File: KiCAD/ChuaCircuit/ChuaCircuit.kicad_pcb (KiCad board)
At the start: 2 copper layers, 30 x 40 mm, 21 parts, among them X1 TP3, Y1 TP2

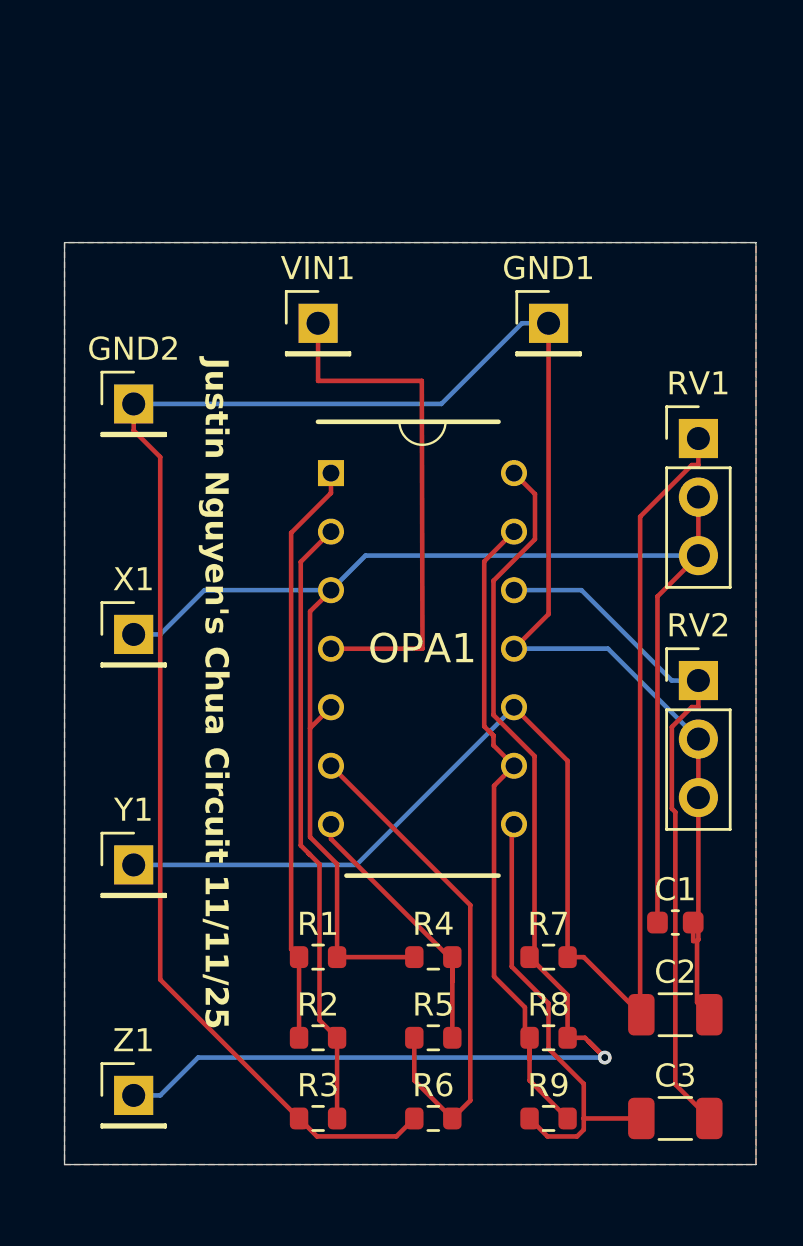
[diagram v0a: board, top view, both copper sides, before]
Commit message: Completed routing and the pcb design but need to make GND plane
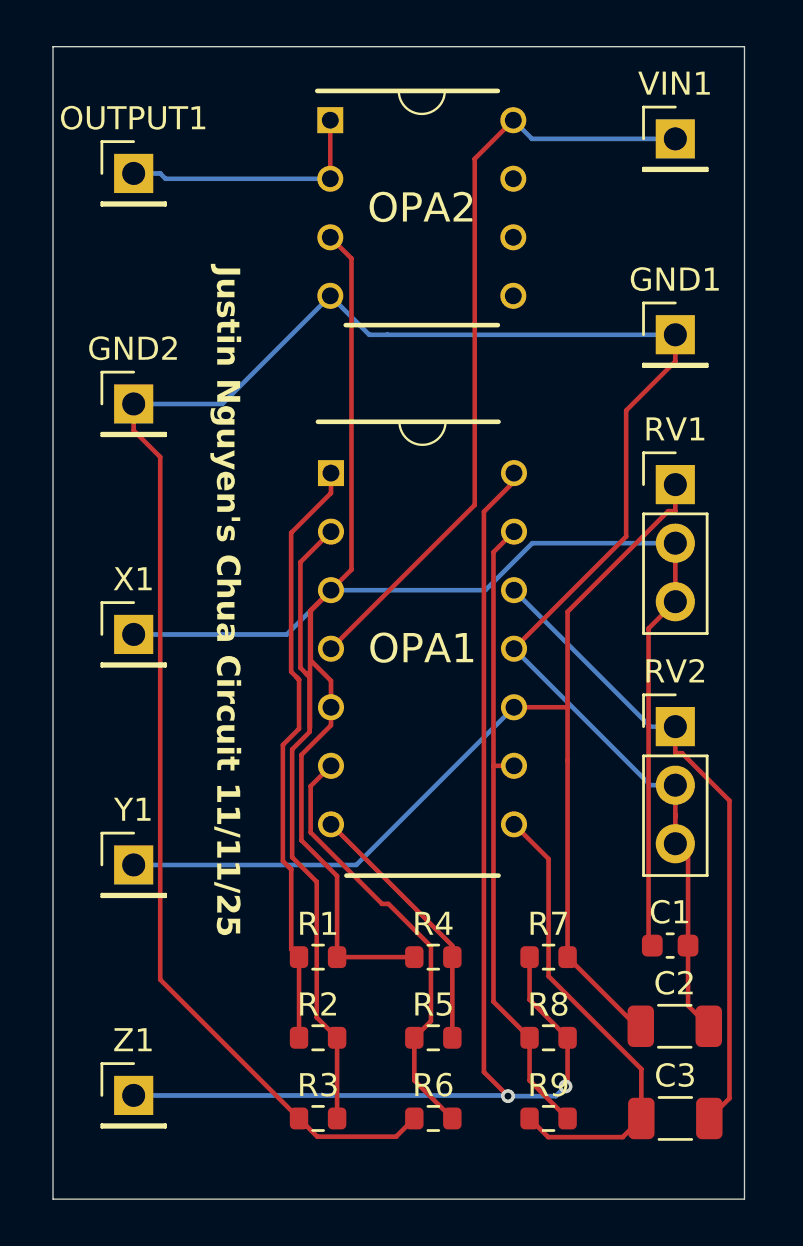
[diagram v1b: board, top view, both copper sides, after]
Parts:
- added OPA2: TL082, SamacSys_Parts:TL082, F.Cu at (138.5, 83.5)
- added OUTPUT1: Male_Header_1x1, Connector_PinHeader_2.54mm:PinHeader_1x01_P2.54mm_Vertical, F.Cu at (126.0, 82.0)
- moved VIN1 17.4 mm to (149.5, 80.5)
- moved GND1 5.52 mm to (149.5, 89.0)
- moved RV1 2.24 mm to (149.5, 95.5)
- moved RV2 2.24 mm to (149.5, 106.0)
- moved C1 1.02 mm to (149.3, 115.5)
- moved C2 0.50 mm to (149.5, 119.0)
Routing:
- net VCC: track 0.00 -> 33.6 mm
- net Net-(OPA1A-+): track 60.2 -> 80.4 mm
- net Net-(OPA1C-+): track 61.5 -> 48.7 mm
- net Net-(OPA2A--): track 0.00 -> 11.2 mm
- net GND: track 96.6 -> 102.8 mm
- net Net-(OPA1B--): track 22.3 -> 19.0 mm
- net Net-(OPA1D-+): track 29.9 -> 28.0 mm
- net Net-(OPA1C--): track 29.4 -> 28.0 mm
- net Net-(OPA1-Pad7): track 12.5 -> 11.4 mm
- net Net-(OPA1-Pad1): track 25.4 -> 26.3 mm
- net Net-(OPA1A--): track 26.8 -> 27.5 mm
- net Net-(C3-Pad1): track 19.9 -> 20.6 mm
- net Net-(OPA1-Pad14): track 54.2 -> 53.8 mm, vias 1 -> 2
- removed copper zone on B.Cu, net GND
- removed copper zone on F.Cu, net GND
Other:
- board size 30 x 40 mm -> 30 x 50 mm
